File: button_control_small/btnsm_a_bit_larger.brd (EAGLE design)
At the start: 19 x 14.9 mm, 18 parts, among them IC1 TINY13V-10SSU, Q1 IRF8788

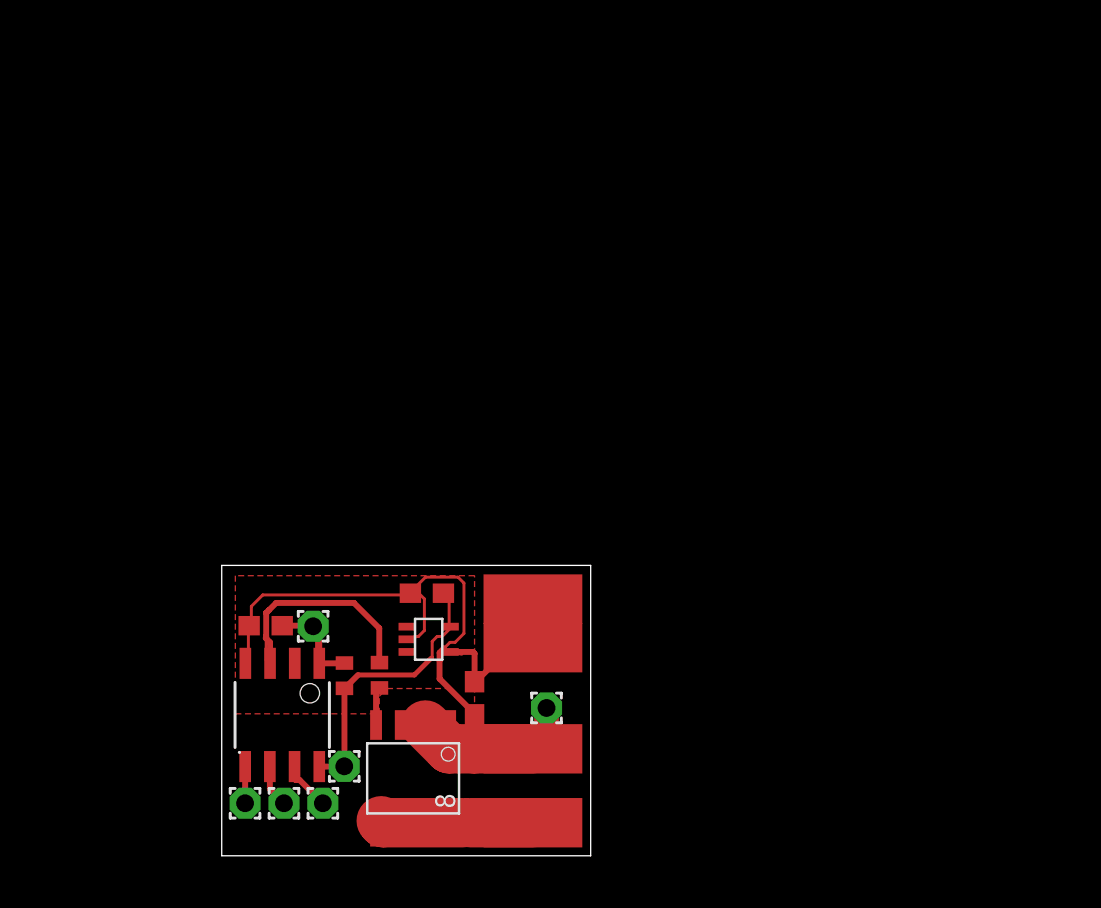
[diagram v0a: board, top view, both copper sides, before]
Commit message: Added version for heater canister
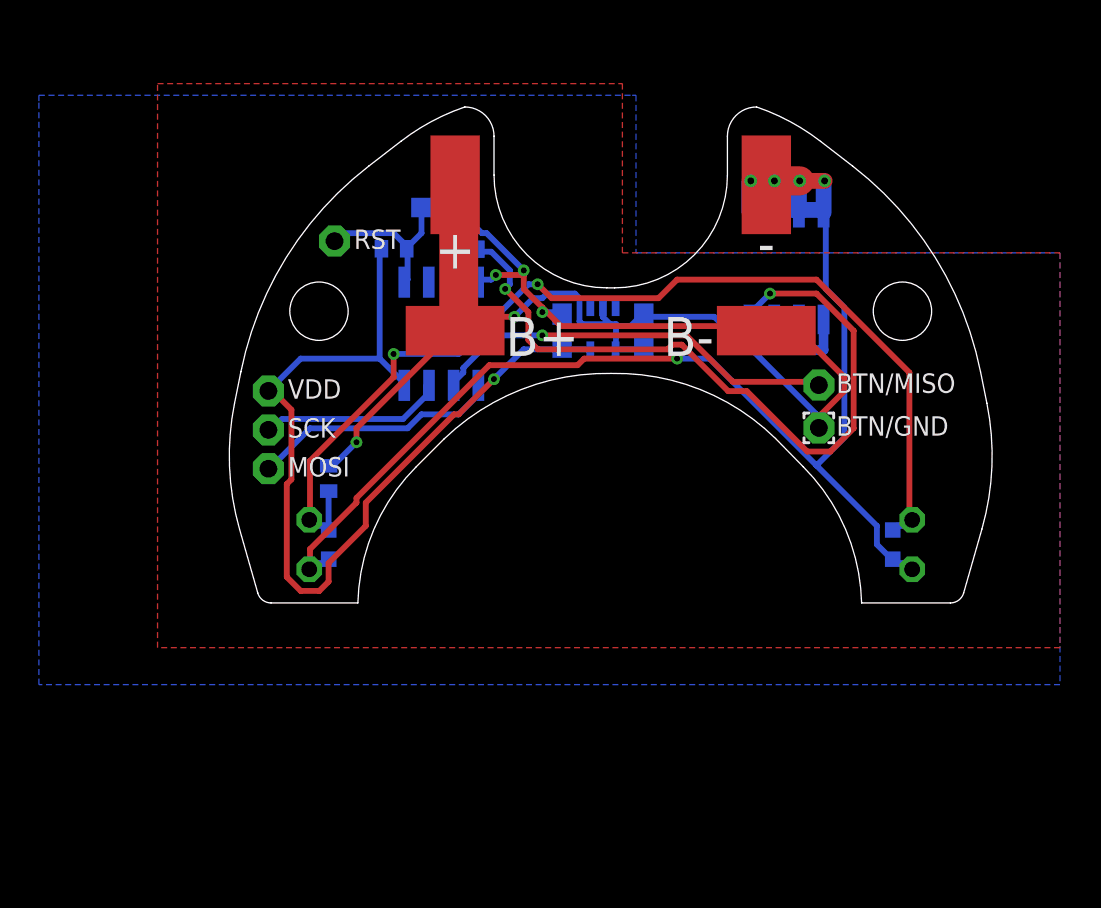
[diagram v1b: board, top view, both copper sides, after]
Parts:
- added LED1, LED3: (no value), eagle-ltspice:LED_SML0603
- added LED2, LED4: (no value), led:LED5MM
- added R3: 300, rcl:R0402
- moved OUT- 34.9 mm to (28.0, 34.5), turned to 180 degrees
- moved PAD2 34.9 mm to (30.7, 24.2), flipped to the bottom
- moved Q1 32.6 mm to (29.0, 30.3), flipped to the bottom, turned to 90 degrees
- moved IN- 24.6 mm to (28.0, 27.0), turned to 90 degrees
- moved C1 23.3 mm to (11.1, 33.3), flipped to the bottom
- moved R1 22.3 mm to (12.5, 31.2), flipped to the bottom, turned to 0 degrees
- moved R2 22.1 mm to (8.86, 31.2), flipped to the bottom, turned to 0 degrees
- moved IN+ 21.7 mm to (12.0, 34.5), turned to 180 degrees
- moved IC1 21.2 mm to (11.3, 26.8), flipped to the bottom
- moved C2 20.8 mm to (21.7, 27.0), flipped to the bottom, turned to 90 degrees
- moved PAD6 20.1 mm to (30.7, 22.0)
- moved PAD4 19.8 mm to (5.80, 31.6), flipped to the bottom
- moved PAD5 19.7 mm to (2.40, 23.9), flipped to the bottom
- moved PAD3 19.4 mm to (2.40, 21.9), flipped to the bottom
- moved U$3 18.3 mm to (19.6, 27.1), flipped to the bottom, turned to 270 degrees
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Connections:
- new net N$6: LED1.A, LED2.A, LED3.A, LED4.A, R3.2
- net N$3: now also R3.1
- net N$4: now also LED1.C, LED2.K, LED3.C, LED4.K
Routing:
- net N$4: track 13.5 -> 71.3 mm, vias 0 -> 5
- net N$6: track 0.00 -> 53.0 mm, vias 0 -> 2
- net N$2: track 2.28 -> 38.0 mm, vias 0 -> 2
- net VDD: track 14.7 -> 46.7 mm, vias 0 -> 1
- net N$3: track 9.79 -> 31.2 mm, vias 0 -> 2
- net MISO: track 2.19 -> 21.1 mm, vias 0 -> 1
- net GND: track 42.6 -> 57.9 mm, vias 0 -> 3
- net N$1: track 12.7 -> 1.72 mm
- net MOSI: track 1.89 -> 12.8 mm
- net SCK: track 2.64 -> 9.45 mm
- added copper zone on layer 16, net GND
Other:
- board size 19 x 14.9 mm -> 39.2 x 25.5 mm
- board text added: "+"
- board text added: "-"
- board text added: "B+"
- board text added: "B-"
- board text added: "BTN/GND"
- board text added: "BTN/MISO"
- board text added: "MOSI"
- board text added: "RST"
- board text added: "SCK"
- board text added: "VDD"

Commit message: Add files via upload
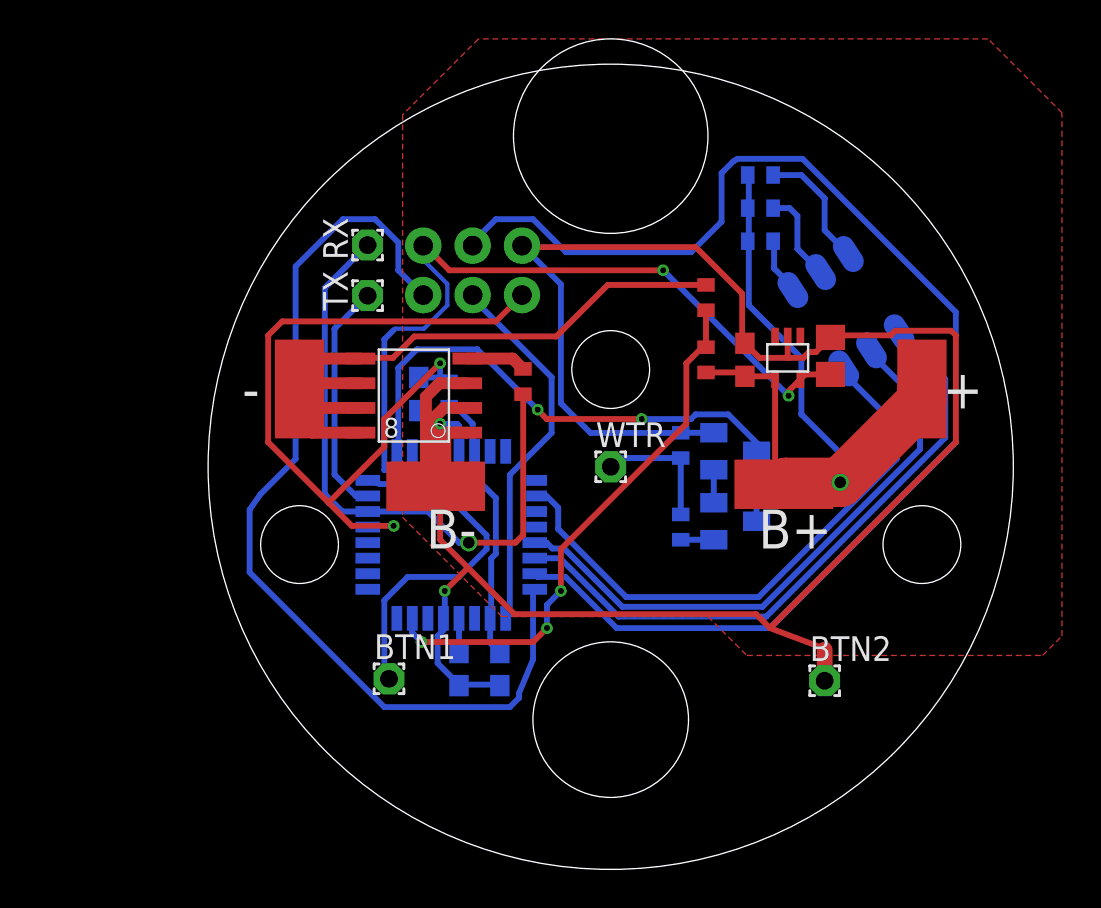
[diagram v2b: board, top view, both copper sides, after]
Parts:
- removed IC1: TINY13V-10SSU, atmel:8S1
- removed LED1, LED3: (no value), eagle-ltspice:LED_SML0603
- removed LED2, LED4: (no value), led:LED5MM
- removed PAD1, PAD2, PAD3, PAD4, PAD5, PAD6: (no value), wirepad:1,6/0,9
- added BTN1: BTN1, wirepad:1,6/0,9
- added BTN2: BNT2, wirepad:1,6/0,9
- added C4, C5: 100n, resistor:C0603
- added D1: (no value), SparkFun-LED:LED-TRICOLOR-5050
- added IC2: MEGA8-AI, atmel:TQFP32-08
- added J1: AVR_SPI_PROG_3X2NS, SparkFun-Connectors:2X3-NS
- added R10: 100k, rcl:R0402
- added R4, R5: 470, rcl:R0402
- added R6: 520, rcl:R0402
- added R7: 282k, rcl:R0402
- added R8: 470k, rcl:R0402
- added R9: 2.2k, rcl:R0402
- added RX: RX, wirepad:1,6/0,9
- added T1, T2: BC848, transistor-neu-to92:SOT23
- added TX: TX, wirepad:1,6/0,9
- added WTR: WATER, wirepad:1,6/0,9
- C2: value 0.33uF -> 100n
- C3: value 2.2uF -> 1uF; device resistor:C0603 -> resistor:C0805
- R3: value 300 -> 100k
- U$3: value TPS71550 -> TPS71533
- moved IN+ 26.2 mm to (36.0, 24.0), turned to 0 degrees
- moved OUT- 26.2 mm to (4.00, 24.0)
- moved R3 21.5 mm to (24.9, 28.7), flipped to the top, turned to 90 degrees
- moved Q1 20.3 mm to (9.88, 23.7), flipped to the top, turned to 180 degrees
- moved IN- 18.8 mm to (11.0, 19.0)
- moved OUT+ 18.7 mm to (28.9, 19.1)
- moved C3 13.9 mm to (31.3, 25.7), flipped to the top
- moved C1 9.64 mm to (10.1, 23.7), turned to 270 degrees
- moved U$3 9.62 mm to (29.1, 25.6), flipped to the top
- moved R2 7.99 mm to (11.7, 23.7), turned to 270 degrees
- moved R1 7.43 mm to (15.5, 24.4), flipped to the top, turned to 270 degrees
- moved C2 5.41 mm to (26.9, 25.5), flipped to the top
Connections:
- removed net N$1: IC1.3, R1.2
- removed net N$3: C2.1, IN+.1, OUT+.1, R3.1, U$3.4
- new net ADC0: IC2.23, R3.1, R7.2
- new net AREF: C5.2, IC2.20
- new net BTN1: BTN1.1, IC2.32
- new net N$13: T1.2, T2.1
- new net N$16: R10.2, R8.1, WTR.1
- new net N$17: R10.1, T1.1
- new net N$18: R9.1, T1.3
- new net N$7: D1.6, R4.2
- new net N$8: D1.4, R5.2
- new net PWM0: D1.3, IC2.10
- new net PWM1: D1.1, IC2.14
- new net PWM2: D1.2, IC2.13
- new net RX: IC2.30, R1.2, RX.1
- new net TX: IC2.31, TX.1
- new net VIN: C2.1, IN+.1, OUT+.1, R4.1, R5.1, R6.1, R7.1, R9.2, U$3.4
- new net WTR: IC2.1, T2.3
- net GND: now also BTN2.1, C4.2, C5.1, IC2.21, IC2.3, IC2.5, J1.6, R8.2, T2.2; no longer IC1.4, PAD6.1
- net MISO: now also IC2.16, J1.1; no longer IC1.6, PAD2.1
- net MOSI: now also IC2.15, J1.4; no longer IC1.5, PAD1.1
- net N$4: now also R3.2; no longer LED1.C, LED2.K, LED3.C, LED4.K
- net N$6: now also D1.5, R6.2; no longer LED1.A, LED2.A, LED3.A, LED4.A, R3.2
- net RST: now also IC2.29, J1.5; no longer IC1.1, PAD4.1
- net SCK: now also IC2.17, J1.3; no longer IC1.7, PAD3.1
- net VDD: now also C4.1, IC2.18, IC2.4, IC2.6, J1.2; no longer IC1.8, PAD5.1
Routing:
- net GND: track 57.9 -> 122.3 mm, vias 3 -> 2
- net MOSI: track 12.8 -> 66.4 mm
- net N$6: track 53.0 -> 4.80 mm, vias 2 -> 0
- net VIN: track 0.00 -> 39.1 mm, vias 0 -> 1
- net N$4: track 71.3 -> 35.5 mm, vias 5 -> 0
- net N$2: track 38.0 -> 3.09 mm, vias 2 -> 0
- net PWM1: track 0.00 -> 32.5 mm
- net RX: track 0.00 -> 32.3 mm, vias 0 -> 1
- net RST: track 8.76 -> 40.9 mm, vias 0 -> 2
- net N$3: track 31.2 -> 0.00 mm, vias 2 -> 0
- net PWM2: track 0.00 -> 30.7 mm
- net PWM0: track 0.00 -> 30.1 mm
- net MISO: track 21.1 -> 49.4 mm, vias 1 -> 0
- net ADC0: track 0.00 -> 28.1 mm, vias 0 -> 3
- net WTR: track 0.00 -> 25.9 mm, vias 0 -> 2
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- removed copper zone on layer 16, net GND
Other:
- board size 39.2 x 25.5 mm -> 41.4 x 41.4 mm
- board text removed: "BTN/GND"
- board text removed: "BTN/MISO"
- board text removed: "MOSI"
- board text removed: "RST"
- board text removed: "SCK"
- board text removed: "VDD"
